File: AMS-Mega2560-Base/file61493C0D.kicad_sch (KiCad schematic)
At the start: 50 parts, among them IC10 LM2597MX-ADJ_NOPB, IC11 LM2597M-3.3_NOPB, IC12 OPA2340PA, IC9 LM2670SX-5.0_NOPB, J21 Screw_Terminal_01x03, J22 Conn_01x07, Q21 IRF9Z34NPBF, Q22 IRF9610PBF-BE3, Q23 2N7000, Q5 2N7000, Q6 IRF9Z34NPBF, U1 BK_HTC-15M, U2 TL431LP

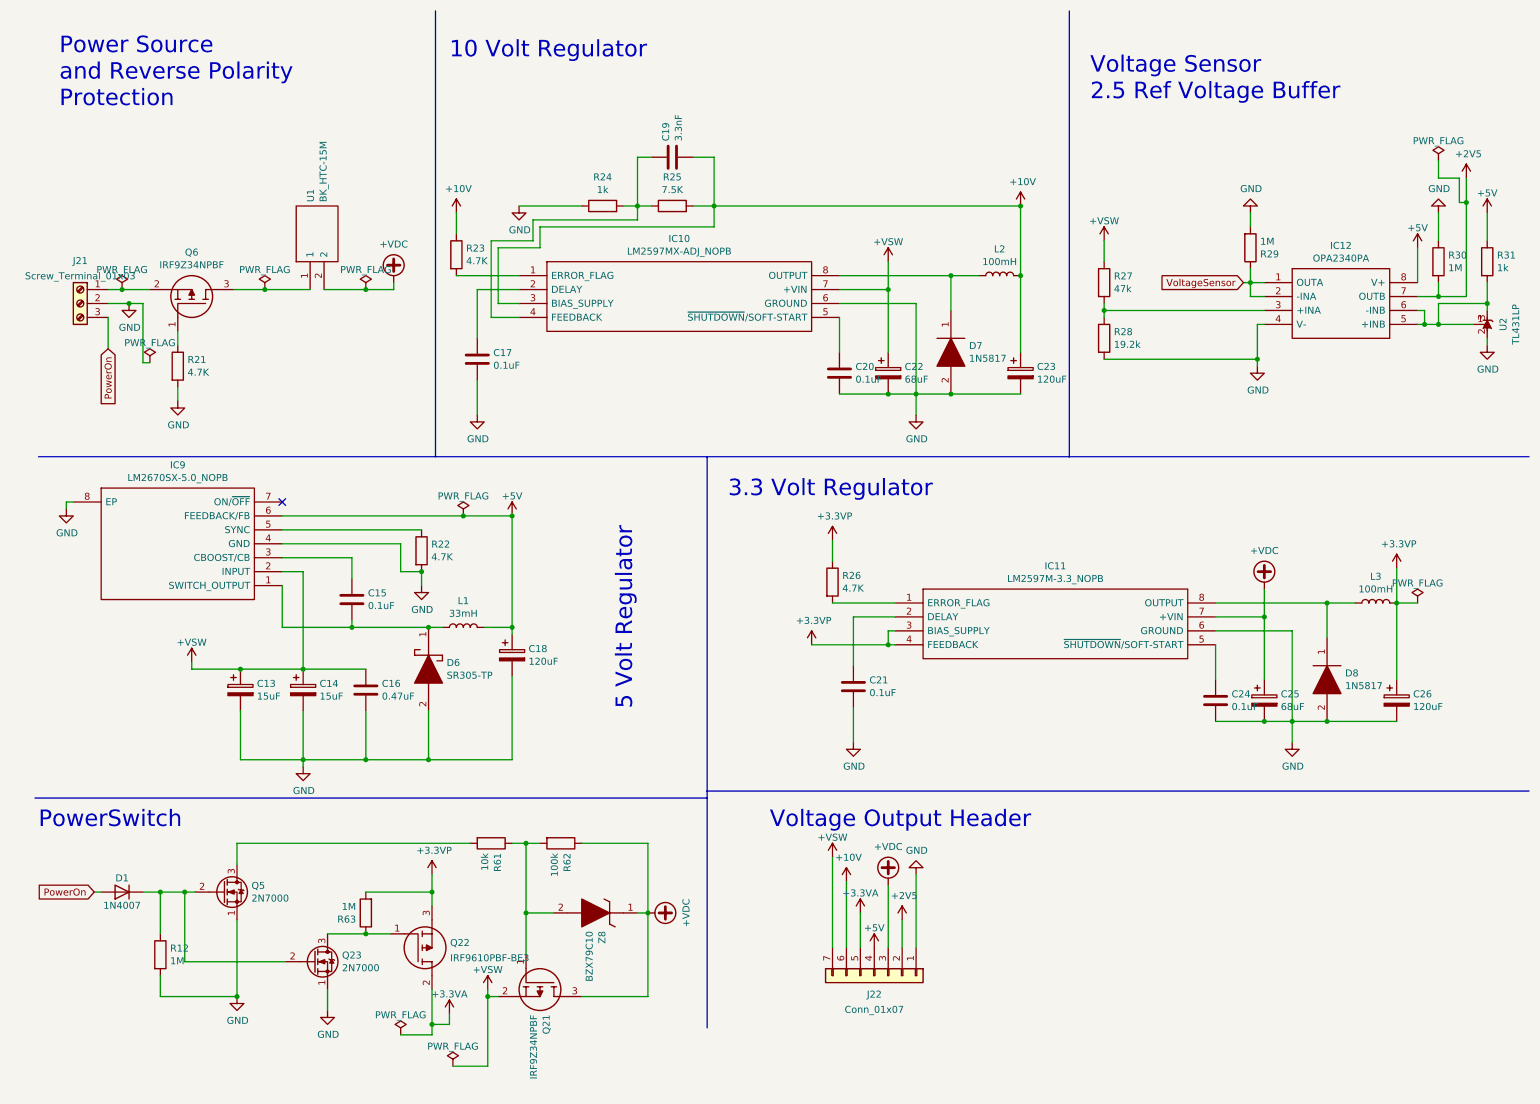
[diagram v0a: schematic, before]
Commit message: working on this.
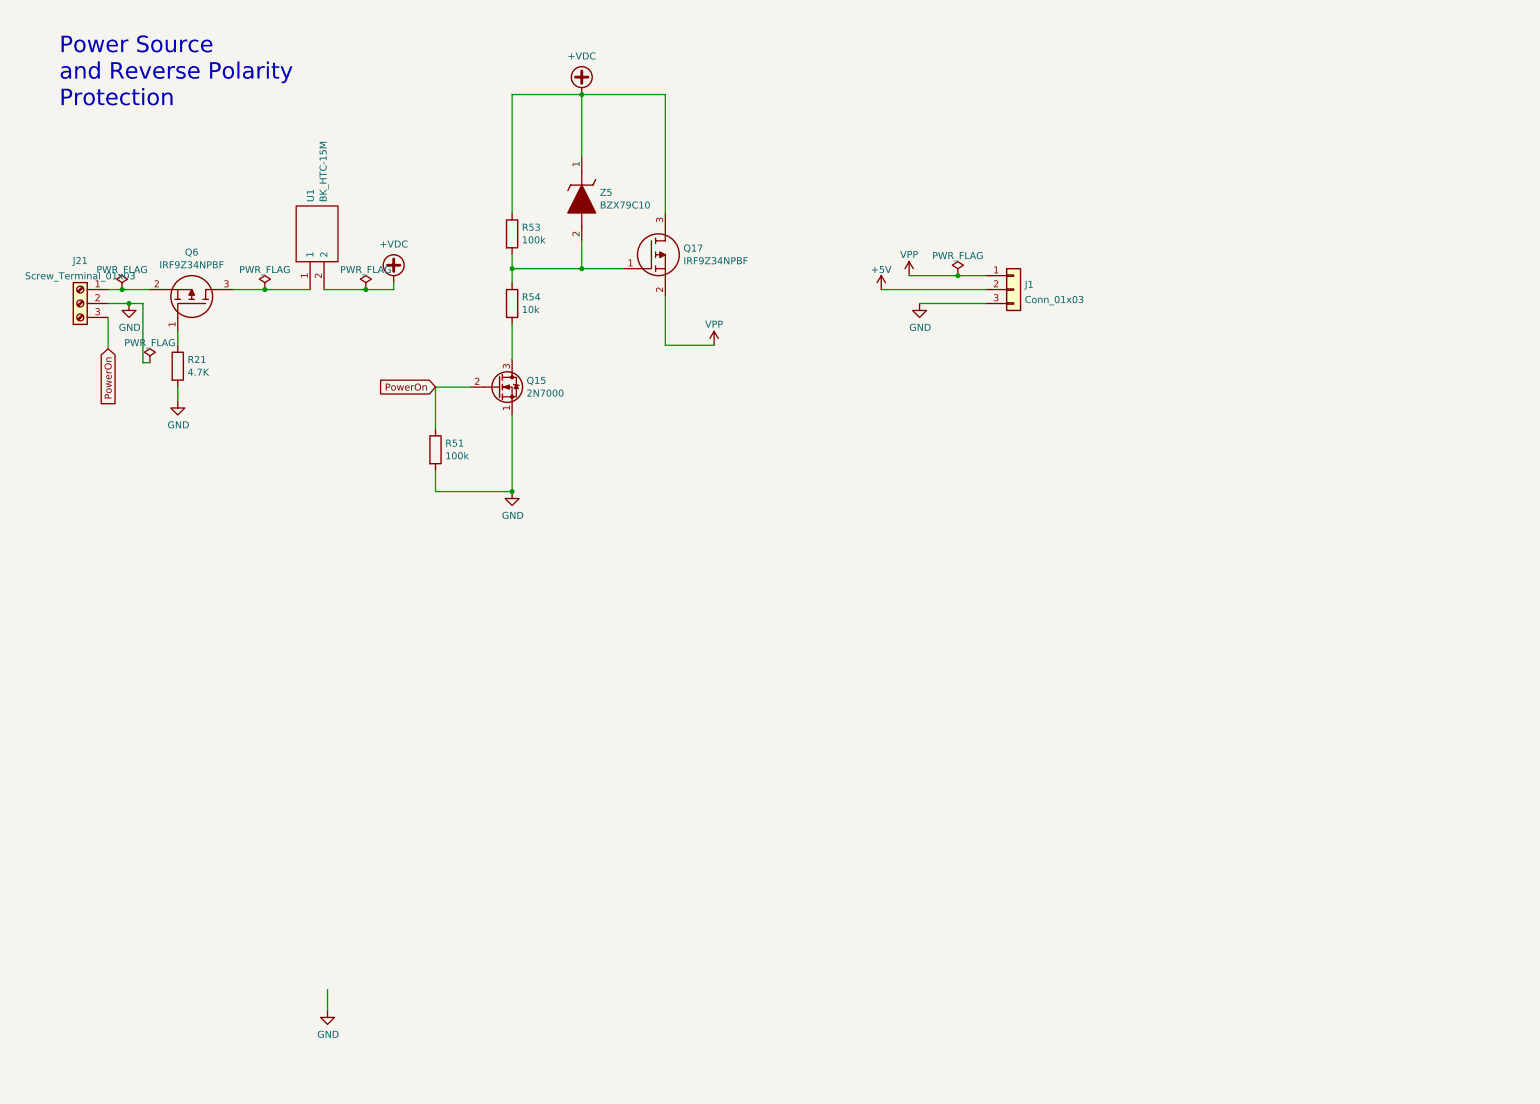
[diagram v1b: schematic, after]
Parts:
- removed C13, C14: 15uF, Capacitor_THT:CP_Radial_D5.0mm_P2.50mm, symbol Device:CP
- removed C15, C17, C20, C21, C24: 0.1uF, Capacitor_THT:C_Rect_L9.0mm_W3.6mm_P7.50mm_MKT, symbol Device:C
- removed C16: 0.47uF, Capacitor_THT:C_Rect_L9.0mm_W3.6mm_P7.50mm_MKT, symbol Device:C
- removed C18, C23, C26: 120uF, Capacitor_THT:CP_Radial_D8.0mm_P5.00mm, symbol Device:CP
- removed C19: 3.3nF, Capacitor_THT:C_Rect_L9.0mm_W3.6mm_P7.50mm_MKT, symbol Device:C
- removed C22, C25: 68uF, Capacitor_THT:CP_Radial_D5.0mm_P2.50mm, symbol Device:CP
- removed D1: 1N4007, Diode_THT:D_DO-41_SOD81_P10.16mm_Horizontal, symbol Diode:1N4007
- removed D6: SR305-TP, SamacSys_Parts:DIOAD2860W130L840D505, symbol SamacSys_Parts:SR305-TP
- removed D7, D8: 1N5817, SamacSys_Parts:DIOAD1414W86L464D238, symbol SamacSys_Parts:1N5817
- removed IC10: LM2597MX-ADJ_NOPB, SamacSys_Parts:SOIC127P600X175-8N, symbol SamacSys_Parts:LM2597MX-ADJ_NOPB
- removed IC11: LM2597M-3.3_NOPB, SamacSys_Parts:SOIC127P600X175-8N, symbol SamacSys_Parts:LM2597M-3.3_NOPB
- removed IC12: OPA2340PA, SamacSys_Parts:DIP794W53P254L959H508Q8N, symbol SamacSys_Parts:OPA2340PA
- removed IC9: LM2670SX-5.0_NOPB, SamacSys_Parts:LM2670SX50NOPB, symbol SamacSys_Parts:LM2670SX-5.0_NOPB
- removed J22: Conn_01x07, Connector_PinHeader_2.54mm:PinHeader_1x07_P2.54mm_Vertical, symbol Connector_Generic:Conn_01x07
- removed L1: 33mH, Inductor_THT:L_Axial_L9.5mm_D4.0mm_P15.24mm_Horizontal_Fastron_SMCC, symbol Device:L
- removed L2, L3: 100mH, Inductor_THT:L_Axial_L9.5mm_D4.0mm_P15.24mm_Horizontal_Fastron_SMCC, symbol Device:L
- removed Q21: IRF9Z34NPBF, SamacSys_Parts:TO254P469X1042X1967-3P, symbol SamacSys_Parts:IRF9Z34NPBF
- removed Q22: IRF9610PBF-BE3, TO254P465X1024X2050-3P, symbol Samac_Sys:IRF9610PBF-BE3
- removed Q23, Q5: 2N7000, Package_TO_SOT_THT:TO-92_Inline, symbol Transistor_FET:2N7000
- removed R12, R29, R30, R63: 1M, Resistor_THT:R_Axial_DIN0207_L6.3mm_D2.5mm_P2.54mm_Vertical, symbol Device:R
- removed R22, R23, R26: 4.7K, Resistor_THT:R_Axial_DIN0207_L6.3mm_D2.5mm_P2.54mm_Vertical, symbol Device:R
- removed R24, R31: 1k, Resistor_THT:R_Axial_DIN0207_L6.3mm_D2.5mm_P2.54mm_Vertical, symbol Device:R
- removed R25: 7.5K, Resistor_THT:R_Axial_DIN0207_L6.3mm_D2.5mm_P2.54mm_Vertical, symbol Device:R
- removed R27: 47k, Resistor_THT:R_Axial_DIN0207_L6.3mm_D2.5mm_P2.54mm_Vertical, symbol Device:R
- removed R28: 19.2k, Resistor_THT:R_Axial_DIN0207_L6.3mm_D2.5mm_P2.54mm_Vertical, symbol Device:R
- removed R61: 10k, Resistor_THT:R_Axial_DIN0207_L6.3mm_D2.5mm_P2.54mm_Vertical, symbol Device:R
- removed R62: 100k, Resistor_THT:R_Axial_DIN0207_L6.3mm_D2.5mm_P2.54mm_Vertical, symbol Device:R
- removed U2: TL431LP, Package_TO_SOT_THT:TO-92_Inline, symbol Reference_Voltage:TL431LP
- removed Z8: BZX79C10, SamacSys_Parts:DIOAD1068W53L380D172, symbol SamacSys_Parts:BZX79C10
- added J1: Conn_01x03, Connector_PinHeader_2.54mm:PinHeader_1x03_P2.54mm_Vertical, symbol Connector_Generic:Conn_01x03
- added Q15: 2N7000, Package_TO_SOT_THT:TO-92_Inline, symbol Transistor_FET:2N7000
- added Q17: IRF9Z34NPBF, SamacSys_Parts:TO254P469X1042X1967-3P, symbol SamacSys_Parts:IRF9Z34NPBF
- added R51, R53: 100k, Resistor_THT:R_Axial_DIN0207_L6.3mm_D2.5mm_P2.54mm_Vertical, symbol Device:R
- added R54: 10k, Resistor_THT:R_Axial_DIN0207_L6.3mm_D2.5mm_P2.54mm_Vertical, symbol Device:R
- added Z5: BZX79C10, SamacSys_Parts:DIOAD1068W53L380D172, symbol SamacSys_Parts:BZX79C10
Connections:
- net +5V: now also J1.2 (Pin_2)
- net +VDC: now also Q17.3, R53.1, Z5.1
- net GND: now also J1.3 (Pin_3), Q15.1 (S), R51.2
- net PowerOn: now also Q15.2 (G), R51.1
- new net: Q17.1, R53.2, R54.1, Z5.2
- new net: Q15.3 (D), R54.2
- new net VPP: J1.1 (Pin_1), Q17.2
- no-connect marks 1 -> 0
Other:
- note removed: "10 Volt Regulator"
- note removed: "3.3 Volt Regulator"
- note removed: "5 Volt Regulator"
- note removed: "PowerSwitch"
- note removed: "Voltage Output Header"
- note removed: "Voltage Sensor 2.5 Ref Voltage Buffer"
